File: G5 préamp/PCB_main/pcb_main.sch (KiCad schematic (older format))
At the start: 47 parts, among them J1 PSU_TUBE, J2 PCB_TUBE, J3 PSU_AMP, J4 AMP, J5 PSU_SIMCAB, J6 SIMCAB, J8 LEVEL 3-2, SW1 Boost, SW2 SIMCAB

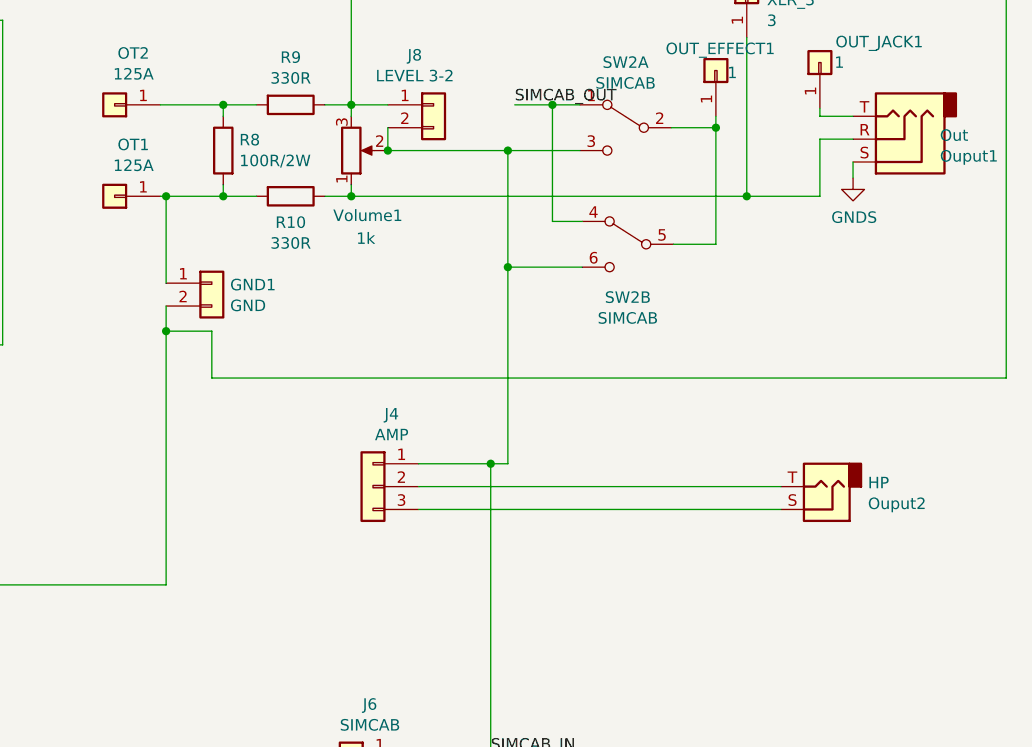
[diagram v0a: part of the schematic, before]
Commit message: Add files via upload
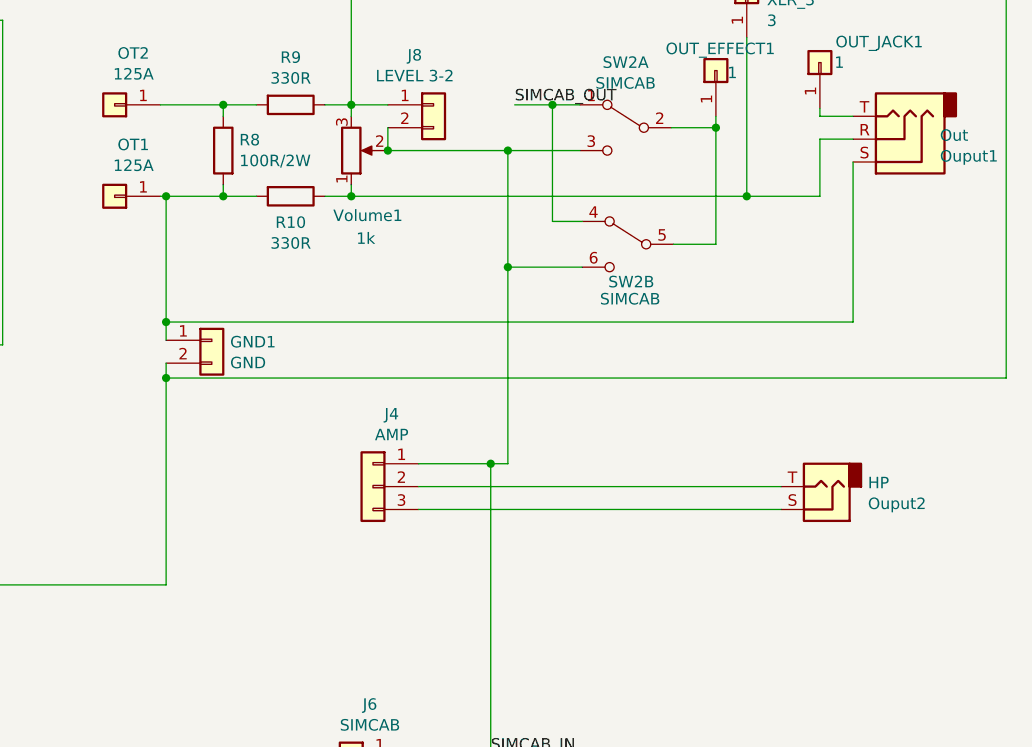
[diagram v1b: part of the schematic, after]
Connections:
- net GNDS: no longer Ouput1.S
- net at GND1.1 (Pin_1), OT1.1 (Pin_1), R10.2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: now also Ouput1.S
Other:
- moved on the sheet: GND1
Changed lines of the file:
@@
 	11060 1355 11060 3025
-Wire Wire Line
-	7585 3025 7585 2820
 Wire Wire Line
 	7360 1830 7635 1830
@@
 L Connector_Generic:Conn_01x02 GND1
 U 1 1 5CB74B24
-P 7585 2610
-F 0 "GND1" H 7665 2602 50  0000 L CNN
-F 1 "GND" H 7665 2511 50  0000 L CNN
-F 2 "Connector_Wire:SolderWirePad_1x02_P7.62mm_Drill2mm" H 7585 2610 50  0001 C CNN
-F 3 "~" H 7585 2610 50  0001 C CNN
-	1    7585 2610
-	1    0    0    -1
-$EndComp
-Wire Wire Line
-	7385 2610 7385 2230
+P 7585 2860
+F 0 "GND1" H 7665 2852 50  0000 L CNN
+F 1 "GND" H 7665 2761 50  0000 L CNN
+F 2 "Connector_Wire:SolderWirePad_1x02_P7.62mm_Drill2mm" H 7585 2860 50  0001 C CNN
+F 3 "~" H 7585 2860 50  0001 C CNN
+	1    7585 2860
+	1    0    0    -1
+$EndComp
+Wire Wire Line
+	7385 2860 7385 2780
 Wire Wire Line
 	5590 2280 5645 2280
@@
 	4740 2780 4780 2780
 Wire Wire Line
-	7385 2710 7385 2820
-Wire Wire Line
-	7585 2820 7385 2820
-Connection ~ 7385 2820
-Wire Wire Line
-	7385 2820 7385 3930
+	7385 2960 7385 3025
+Connection ~ 7385 3025
+Wire Wire Line
+	7385 3025 7385 3930
 Wire Wire Line
 	2035 5125 2480 5125
@@
 Wire Wire Line
 	8345 2030 8355 2030
-Wire Wire Line
-	7585 3025 11060 3025
 $Comp
 L Connector_Generic:Conn_01x01 OUT_EFFECT1
@@
 U 2 1 5CB34261
 P 9405 2440
-F 0 "SW2" H 9405 2207 50  0000 C CNN
-F 1 "SIMCAB" H 9405 2116 50  0000 C CNN
+F 0 "SW2" H 9390 2275 50  0000 C CNN
+F 1 "SIMCAB" H 9395 2200 50  0000 C CNN
 F 2 "Switch_lever:SW_CK_Lever_DPDT_72xx" H 9405 2440 50  0001 C CNN
 F 3 "~" H 9405 2440 50  0001 C CNN
@@
 Text Label 4060 1460 0    50   ~ 0
 G_V2
-$Comp
-L power:GNDS #PWR0105
-U 1 1 5CAB190D
-P 10390 2150
-F 0 "#PWR0105" H 10390 1900 50  0001 C CNN
-F 1 "GNDS" H 10395 1977 50  0000 C CNN
-F 2 "" H 10390 2150 50  0001 C CNN
-F 3 "" H 10390 2150 50  0001 C CNN
-	1    10390 2150
-	1    0    0    -1
-$EndComp
-Wire Wire Line
-	10390 2080 10390 2150
 Wire Wire Line
 	10245 1980 10245 2230
 Wire Wire Line
 	10245 1980 10390 1980
+Wire Wire Line
+	7385 3025 11060 3025
+Wire Wire Line
+	7385 2780 10390 2780
+Wire Wire Line
+	10390 2780 10390 2080
+Connection ~ 7385 2780
+Wire Wire Line
+	7385 2780 7385 2230
 $EndSCHEMATC
